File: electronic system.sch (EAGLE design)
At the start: 63 parts, among them IC1 TDA2040V, IC2 TDA2040V, IC3 TDA2040V, IC4 TDA2040V

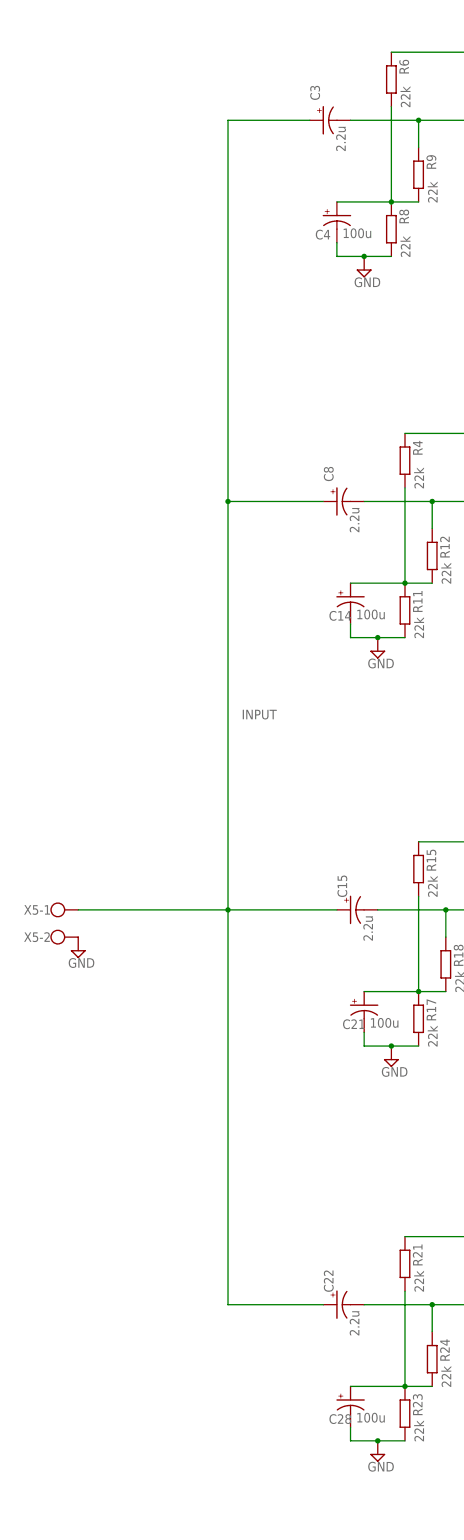
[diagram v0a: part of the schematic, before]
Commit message: First schematic
Developing
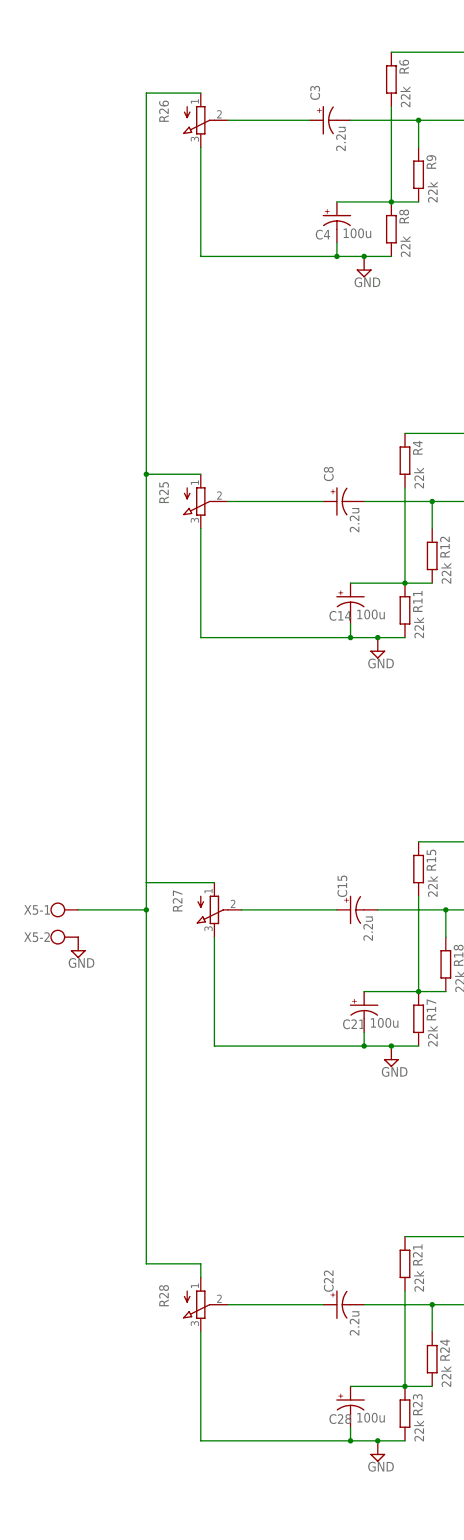
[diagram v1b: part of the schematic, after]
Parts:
- added R25, R26, R27, R28: (no value), pot:3RP/1610N
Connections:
- new net N$25: C22.+, R28.S
- new net N$27: C3.+, R26.S
- new net N$29: R25.A, R26.A, R27.A, R28.A, X5-1.KL
- new net N$30: C15.+, R27.S
- net GND: now also R25.E, R26.E, R27.E, R28.E
- net INPUT: now also R25.S; no longer C15.+, C22.+, C3.+, X5-1.KL
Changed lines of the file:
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@@
 <part name="SUPPLY25" library="supply2" library_urn="urn:adsk.eagle:library:372" deviceset="GND" device=""/>
 <part name="SUPPLY26" library="supply2" library_urn="urn:adsk.eagle:library:372" deviceset="GND" device=""/>
+<part name="R25" library="pot" library_urn="urn:adsk.eagle:library:331" deviceset="3RP/1610N" device="" package3d_urn="urn:adsk.eagle:package:22726/1"/>
+<part name="R26" library="pot" library_urn="urn:adsk.eagle:library:331" deviceset="3RP/1610N" device="" package3d_urn="urn:adsk.eagle:package:22726/1"/>
+<part name="R27" library="pot" library_urn="urn:adsk.eagle:library:331" deviceset="3RP/1610N" device="" package3d_urn="urn:adsk.eagle:package:22726/1"/>
+<part name="R28" library="pot" library_urn="urn:adsk.eagle:library:331" deviceset="3RP/1610N" device="" package3d_urn="urn:adsk.eagle:package:22726/1"/>
 </parts>
 <sheets>
@@
 <instance part="SUPPLY26" gate="GND" x="7.62" y="-27.94" smashed="yes">
 <attribute name="VALUE" x="5.715" y="-31.115" size="1.778" layer="96"/>
+</instance>
+<instance part="R25" gate="G$1" x="30.48" y="55.88" smashed="yes" rot="MR180">
+<attribute name="NAME" x="24.511" y="59.69" size="1.778" layer="95" rot="MR270"/>
+<attribute name="VALUE" x="26.67" y="59.69" size="1.778" layer="96" rot="MR270"/>
+</instance>
+<instance part="R26" gate="G$1" x="30.48" y="127" smashed="yes" rot="MR180">
+<attribute name="NAME" x="24.511" y="130.81" size="1.778" layer="95" rot="MR270"/>
+<attribute name="VALUE" x="26.67" y="130.81" size="1.778" layer="96" rot="MR270"/>
+</instance>
+<instance part="R27" gate="G$1" x="33.02" y="-20.32" smashed="yes" rot="MR180">
+<attribute name="NAME" x="27.051" y="-16.51" size="1.778" layer="95" rot="MR270"/>
+<attribute name="VALUE" x="29.21" y="-16.51" size="1.778" layer="96" rot="MR270"/>
+</instance>
+<instance part="R28" gate="G$1" x="30.48" y="-93.98" smashed="yes" rot="MR180">
+<attribute name="NAME" x="24.511" y="-90.17" size="1.778" layer="95" rot="MR270"/>
+<attribute name="VALUE" x="26.67" y="-90.17" size="1.778" layer="96" rot="MR270"/>
 </instance>
 </instances>
@@
 <pinref part="R8" gate="G$1" pin="2"/>
 <wire x1="55.88" y1="104.14" x2="55.88" y2="101.6" width="0.1524" layer="91"/>
+<pinref part="SUPPLY2" gate="GND" pin="GND"/>
 <wire x1="55.88" y1="101.6" x2="60.96" y2="101.6" width="0.1524" layer="91"/>
-<pinref part="SUPPLY2" gate="GND" pin="GND"/>
 <wire x1="60.96" y1="101.6" x2="66.04" y2="101.6" width="0.1524" layer="91"/>
 <junction x="60.96" y="101.6"/>
 <pinref part="C4" gate="G$1" pin="-"/>
+<pinref part="R26" gate="G$1" pin="E"/>
+<wire x1="30.48" y1="121.92" x2="30.48" y2="101.6" width="0.1524" layer="91"/>
+<wire x1="30.48" y1="101.6" x2="55.88" y2="101.6" width="0.1524" layer="91"/>
+<junction x="55.88" y="101.6"/>
 </segment>
 <segment>
@@
 <junction x="63.5" y="30.48"/>
 <pinref part="C14" gate="G$1" pin="-"/>
+<pinref part="R25" gate="G$1" pin="E"/>
+<wire x1="30.48" y1="50.8" x2="30.48" y2="30.48" width="0.1524" layer="91"/>
+<wire x1="30.48" y1="30.48" x2="58.42" y2="30.48" width="0.1524" layer="91"/>
+<junction x="58.42" y="30.48"/>
 </segment>
 <segment>
@@
 <junction x="66.04" y="-45.72"/>
 <pinref part="C21" gate="G$1" pin="-"/>
+<pinref part="R27" gate="G$1" pin="E"/>
+<wire x1="60.96" y1="-45.72" x2="33.02" y2="-45.72" width="0.1524" layer="91"/>
+<wire x1="33.02" y1="-45.72" x2="33.02" y2="-25.4" width="0.1524" layer="91"/>
+<junction x="60.96" y="-45.72"/>
 </segment>
 <segment>
@@
 <junction x="63.5" y="-119.38"/>
 <pinref part="C28" gate="G$1" pin="-"/>
+<pinref part="R28" gate="G$1" pin="E"/>
+<wire x1="30.48" y1="-99.06" x2="30.48" y2="-119.38" width="0.1524" layer="91"/>
+<wire x1="30.48" y1="-119.38" x2="58.42" y2="-119.38" width="0.1524" layer="91"/>
+<junction x="58.42" y="-119.38"/>
 </segment>
 <segment>
@@
 <net name="INPUT" class="0">
 <segment>
-<pinref part="C22" gate="G$1" pin="+"/>
-<wire x1="53.34" y1="-93.98" x2="35.56" y2="-93.98" width="0.1524" layer="91"/>
-<pinref part="C15" gate="G$1" pin="+"/>
-<wire x1="35.56" y1="-93.98" x2="35.56" y2="-20.32" width="0.1524" layer="91"/>
-<wire x1="35.56" y1="-20.32" x2="55.88" y2="-20.32" width="0.1524" layer="91"/>
 <pinref part="C8" gate="G$1" pin="+"/>
 <wire x1="53.34" y1="55.88" x2="35.56" y2="55.88" width="0.1524" layer="91"/>
-<wire x1="35.56" y1="55.88" x2="35.56" y2="-20.32" width="0.1524" layer="91"/>
-<junction x="35.56" y="-20.32"/>
-<pinref part="C3" gate="G$1" pin="+"/>
-<wire x1="35.56" y1="55.88" x2="35.56" y2="127" width="0.1524" layer="91"/>
-<wire x1="35.56" y1="127" x2="50.8" y2="127" width="0.1524" layer="91"/>
-<junction x="35.56" y="55.88"/>
-<label x="38.1" y="15.24" size="1.778" layer="95"/>
-<pinref part="X5" gate="-1" pin="KL"/>
-<wire x1="7.62" y1="-20.32" x2="35.56" y2="-20.32" width="0.1524" layer="91"/>
+<pinref part="R25" gate="G$1" pin="S"/>
 </segment>
 </net>
@@
 </segment>
 </net>
+<net name="N$25" class="0">
+<segment>
+<pinref part="C22" gate="G$1" pin="+"/>
+<wire x1="53.34" y1="-93.98" x2="35.56" y2="-93.98" width="0.1524" layer="91"/>
+<pinref part="R28" gate="G$1" pin="S"/>
+</segment>
+</net>
+<net name="N$27" class="0">
+<segment>
+<pinref part="C3" gate="G$1" pin="+"/>
+<wire x1="35.56" y1="127" x2="50.8" y2="127" width="0.1524" layer="91"/>
+<pinref part="R26" gate="G$1" pin="S"/>
+</segment>
+</net>
+<net name="N$29" class="0">
+<segment>
+<pinref part="R27" gate="G$1" pin="A"/>
+<wire x1="20.32" y1="-15.24" x2="33.02" y2="-15.24" width="0.1524" layer="91"/>
+<pinref part="R28" gate="G$1" pin="A"/>
+<wire x1="30.48" y1="-88.9" x2="30.48" y2="-86.36" width="0.1524" layer="91"/>
+<wire x1="30.48" y1="-86.36" x2="20.32" y2="-86.36" width="0.1524" layer="91"/>
+<pinref part="X5" gate="-1" pin="KL"/>
+<wire x1="20.32" y1="-86.36" x2="20.32" y2="-20.32" width="0.1524" layer="91"/>
+<wire x1="20.32" y1="-20.32" x2="7.62" y2="-20.32" width="0.1524" layer="91"/>
+<junction x="20.32" y="-20.32"/>
+<pinref part="R25" gate="G$1" pin="A"/>
+<wire x1="20.32" y1="-15.24" x2="20.32" y2="-20.32" width="0.1524" layer="91"/>
+<wire x1="30.48" y1="60.96" x2="20.32" y2="60.96" width="0.1524" layer="91"/>
+<wire x1="20.32" y1="60.96" x2="20.32" y2="-15.24" width="0.1524" layer="91"/>
+<pinref part="R26" gate="G$1" pin="A"/>
+<wire x1="30.48" y1="132.08" x2="20.32" y2="132.08" width="0.1524" layer="91"/>
+<wire x1="20.32" y1="132.08" x2="20.32" y2="60.96" width="0.1524" layer="91"/>
+<junction x="20.32" y="60.96"/>
+</segment>
+</net>
+<net name="N$30" class="0">
+<segment>
+<pinref part="R27" gate="G$1" pin="S"/>
+<pinref part="C15" gate="G$1" pin="+"/>
+<wire x1="38.1" y1="-20.32" x2="55.88" y2="-20.32" width="0.1524" layer="91"/>
+</segment>
+</net>
